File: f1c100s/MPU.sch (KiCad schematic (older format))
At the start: 31 parts, among them IC1 F1C100S, Y1 Crystal

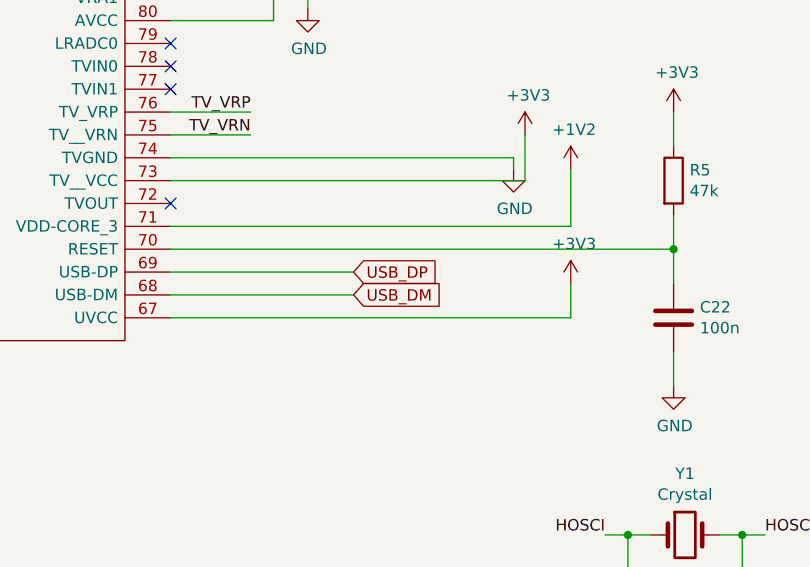
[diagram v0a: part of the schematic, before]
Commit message: All done i guess. DRC a little bit fuzzy but whatever.
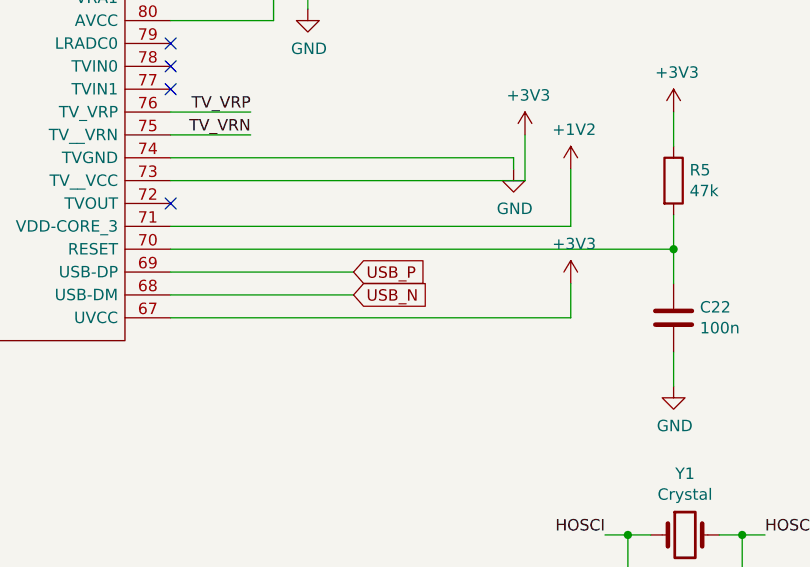
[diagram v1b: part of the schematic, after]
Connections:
- net USB_DM renamed USB_N
- net USB_DP renamed USB_P
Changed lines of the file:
@@
 	6900 2200 6900 2050
 Text GLabel 9000 4500 2    50   Input ~ 0
-USB_DP
+USB_P
 Text GLabel 9000 4600 2    50   Input ~ 0
-USB_DM
+USB_N
 Wire Wire Line
 	8200 4600 9000 4600
